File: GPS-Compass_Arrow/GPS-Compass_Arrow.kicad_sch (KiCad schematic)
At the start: 153 parts, among them IC1 74VHC9595FT, IC2 74VHC9595FT, IC3 74VHC9595FT, IC4 74VHC9595FT, IC5 74VHC9595FT, IC6 74VHC9595FT, IC7 74VHC9595FT, IC8 74VHC9595FT, J1 FFC2B28-12-G, J2 INDICATOR, U1 OSK3056A-LR, U2 MAX7219

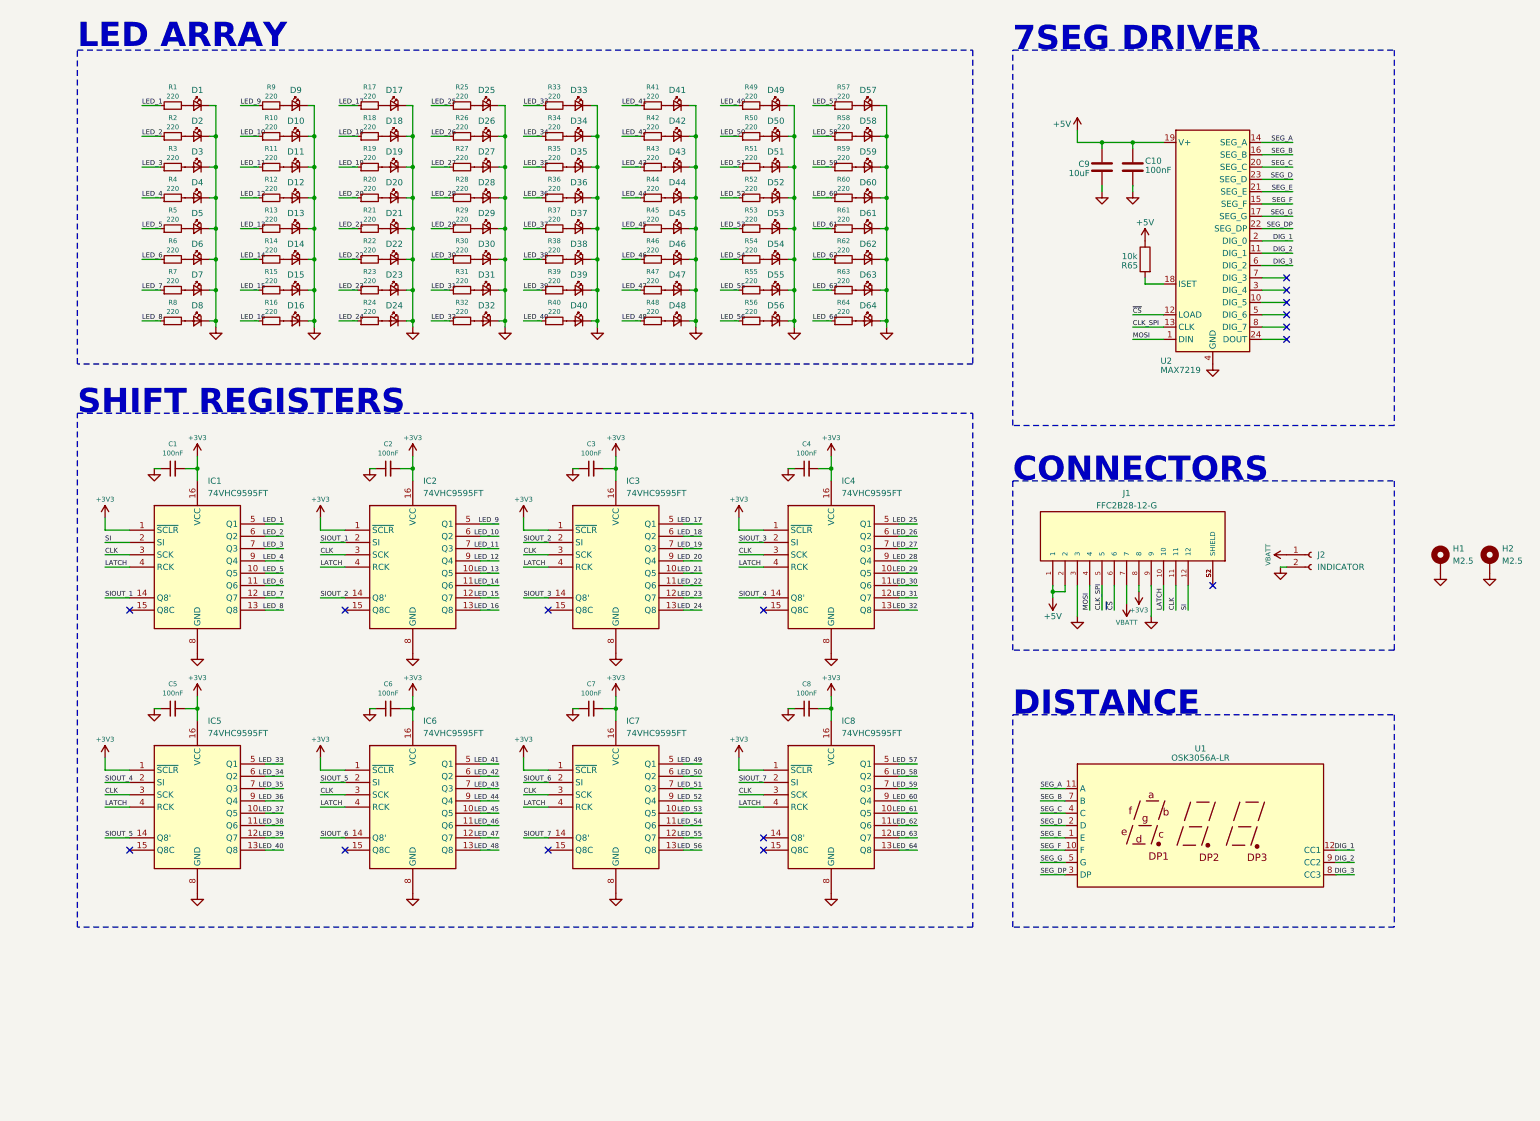
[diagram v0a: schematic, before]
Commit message: main pcb and arrow updatws
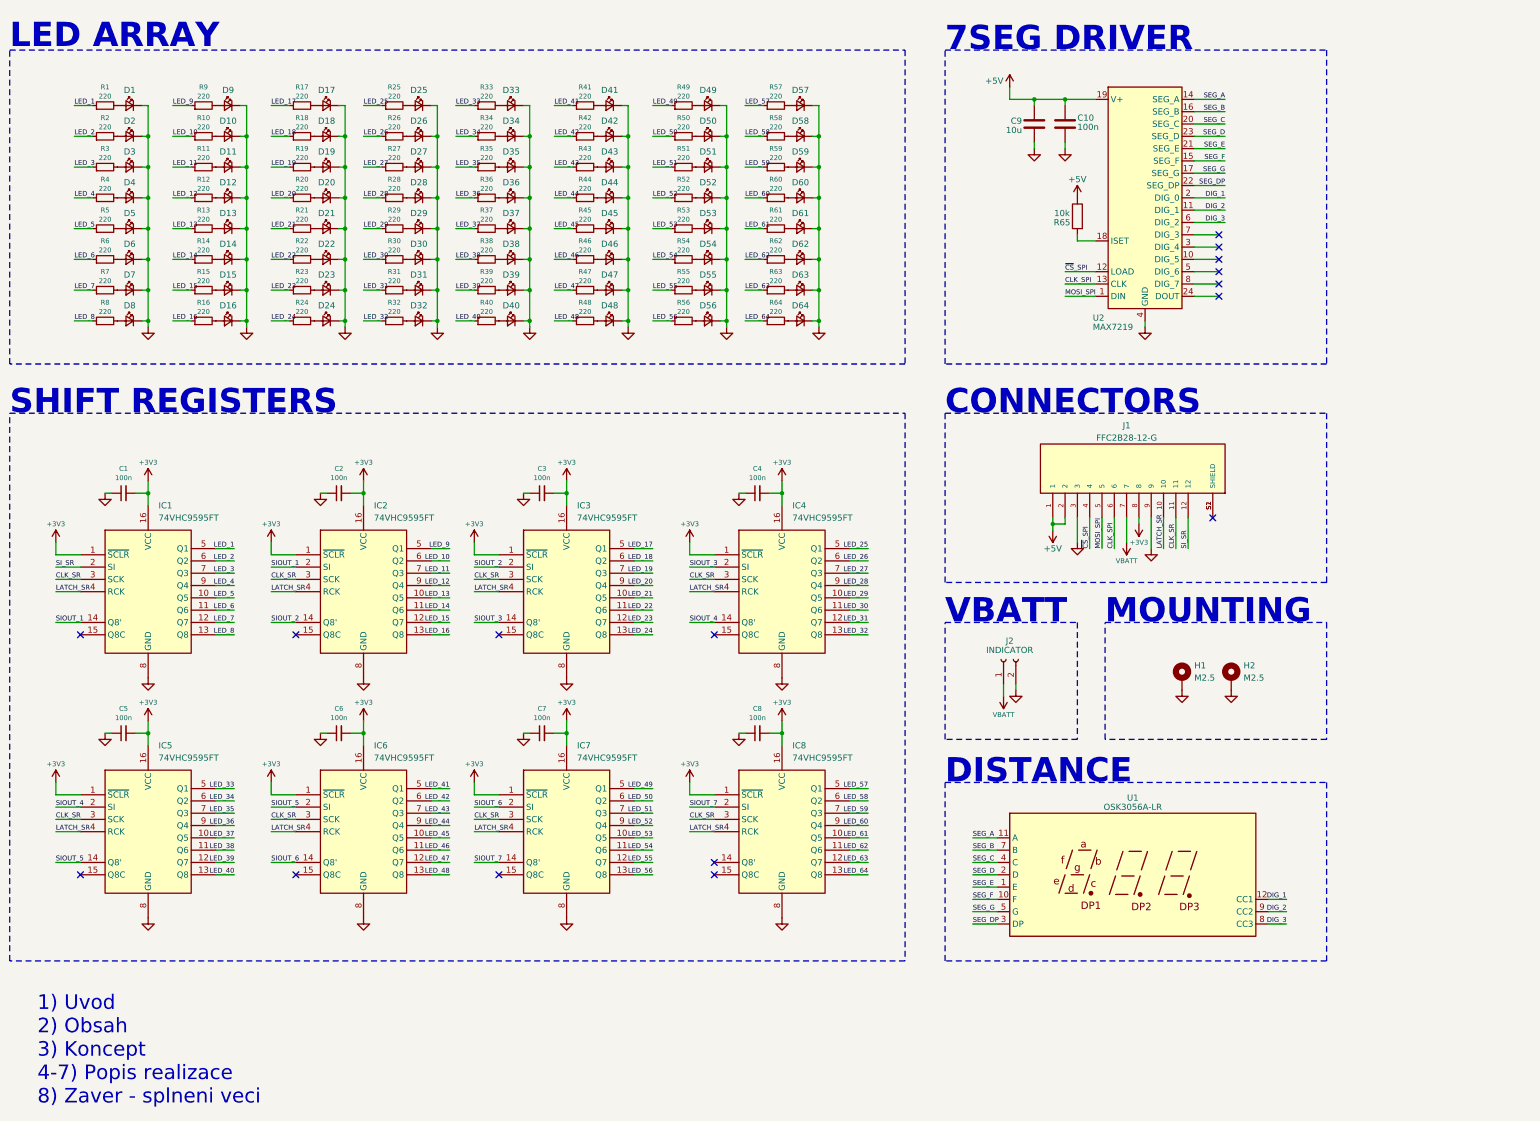
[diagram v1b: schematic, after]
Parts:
- C1, C10, C2, C3, C4, C5, C6, C7, C8: value 100nF -> 100n
- C9: value 10uF -> 10u
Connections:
- net CLK_SPI: now also J1.6; no longer J1.5
- net CLK renamed CLK_SR
- net LATCH renamed LATCH_SR
- net MOSI renamed MOSI_SPI
- net MOSI_SPI: now also J1.5; no longer J1.4
- net SI renamed SI_SR
- net ~{CS} renamed ~{CS}_SPI
- net ~{CS}_SPI: now also J1.4; no longer J1.6
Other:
- note added: "1) Uvod 2) Obsah 3) Koncept 4-7) Popis realizace 8) Zaver - splneni veci"
- note added: "MOUNTING"
- note added: "VBATT"
- moved on the sheet: C1, C10, C2, C3, C4, C5, C6, C7, C8, C9, D1, D10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
